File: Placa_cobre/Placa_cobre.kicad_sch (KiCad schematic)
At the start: 3 parts

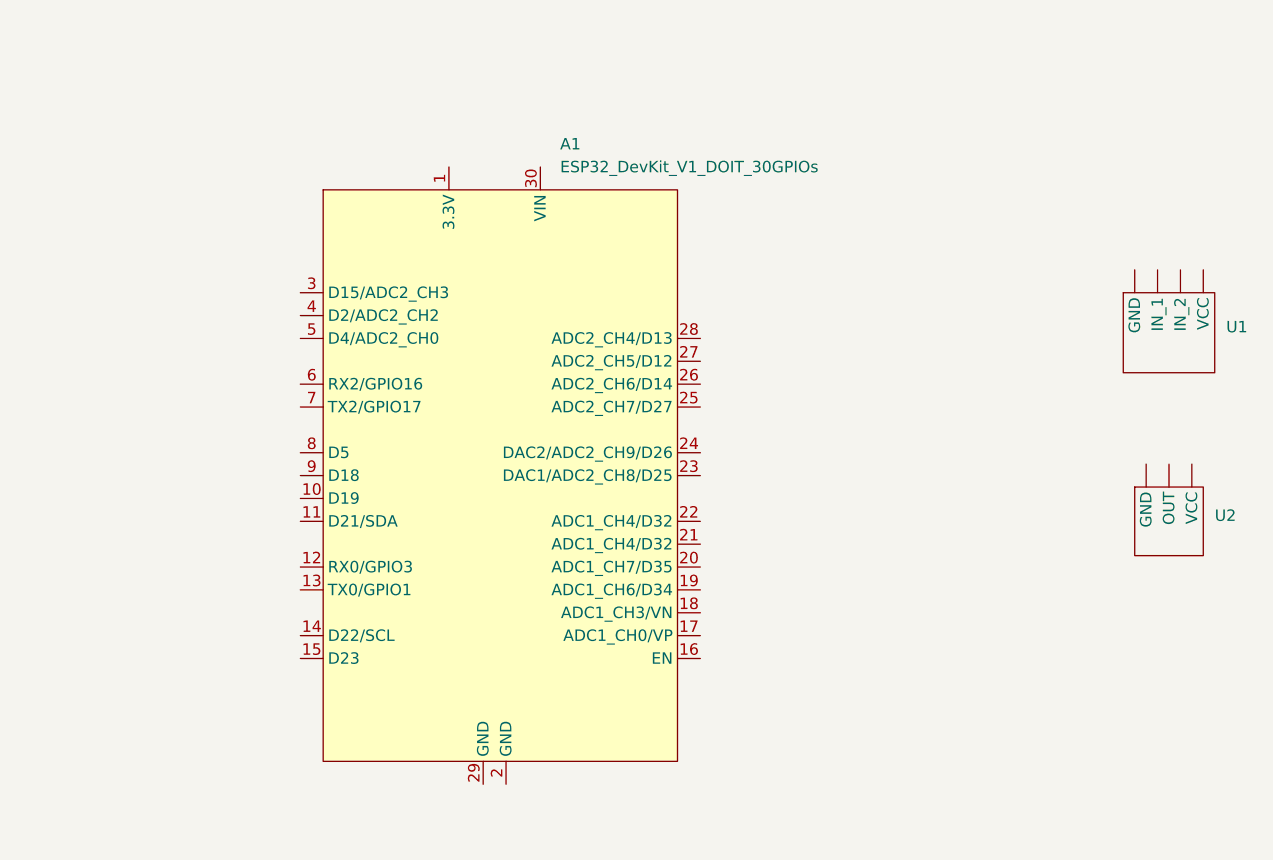
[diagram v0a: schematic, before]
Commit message: codigo funcional, mandando e recebendo sinal, recpetor e transmissor
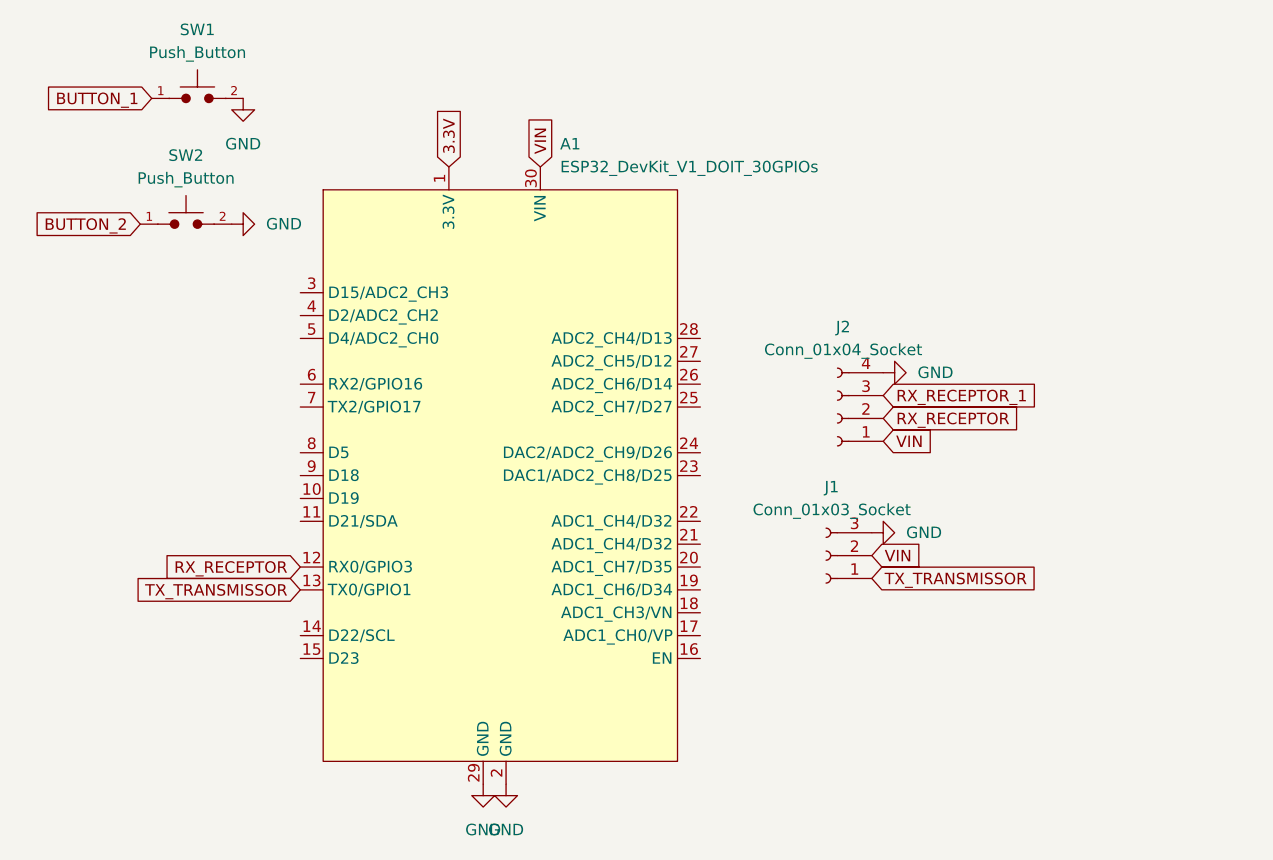
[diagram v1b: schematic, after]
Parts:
- removed U1: ~, symbol RF_transmissor_receptor:RF_RECEPTOR
- removed U2: ~, symbol RF_transmissor_receptor:rf_transmissor
- added J1: Conn_01x03_Socket, Connector_PinSocket_2.54mm:PinSocket_1x03_P2.54mm_Vertical, symbol Connector:Conn_01x03_Socket
- added J2: Conn_01x04_Socket, Connector_PinSocket_2.54mm:PinSocket_1x04_P2.54mm_Vertical, symbol Connector:Conn_01x04_Socket
- added SW1, SW2: Push_Button, Button_Switch_THT:SW_PUSH_6mm, symbol PCM_SL_Devices:Push_Button
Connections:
- net 3.3V: now reaches A1.1 (3.3V)
- net RX_RECEPTOR: now reaches A1.12 (RX0/GPIO3)
- net RX_RECEPTOR: now also J2.2 (Pin_2)
- net TX_TRANSMISSOR: now reaches A1.13 (TX0/GPIO1)
- net TX_TRANSMISSOR: now also J1.1 (Pin_1)
- net GND: now reaches A1.2 (GND)
- net GND: now also A1.29 (GND), J1.3 (Pin_3), J2.4 (Pin_4), SW1.2, SW2.2
- net VIN: now reaches A1.30 (VIN)
- net VIN: now also J1.2 (Pin_2), J2.1 (Pin_1)
- new net BUTTON_1: SW1.1
- new net BUTTON_2: SW2.1
- new net RX_RECEPTOR_1: J2.3 (Pin_3)
